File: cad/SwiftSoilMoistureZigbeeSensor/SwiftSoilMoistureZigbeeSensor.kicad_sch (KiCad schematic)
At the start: 12 parts, among them J1 Probe, J2 BAT, J3 TagConnect, Q1 BSS84, SW1 Factory Reset, U1 TPS61221DCK, U2 E73-2G4M08S1C

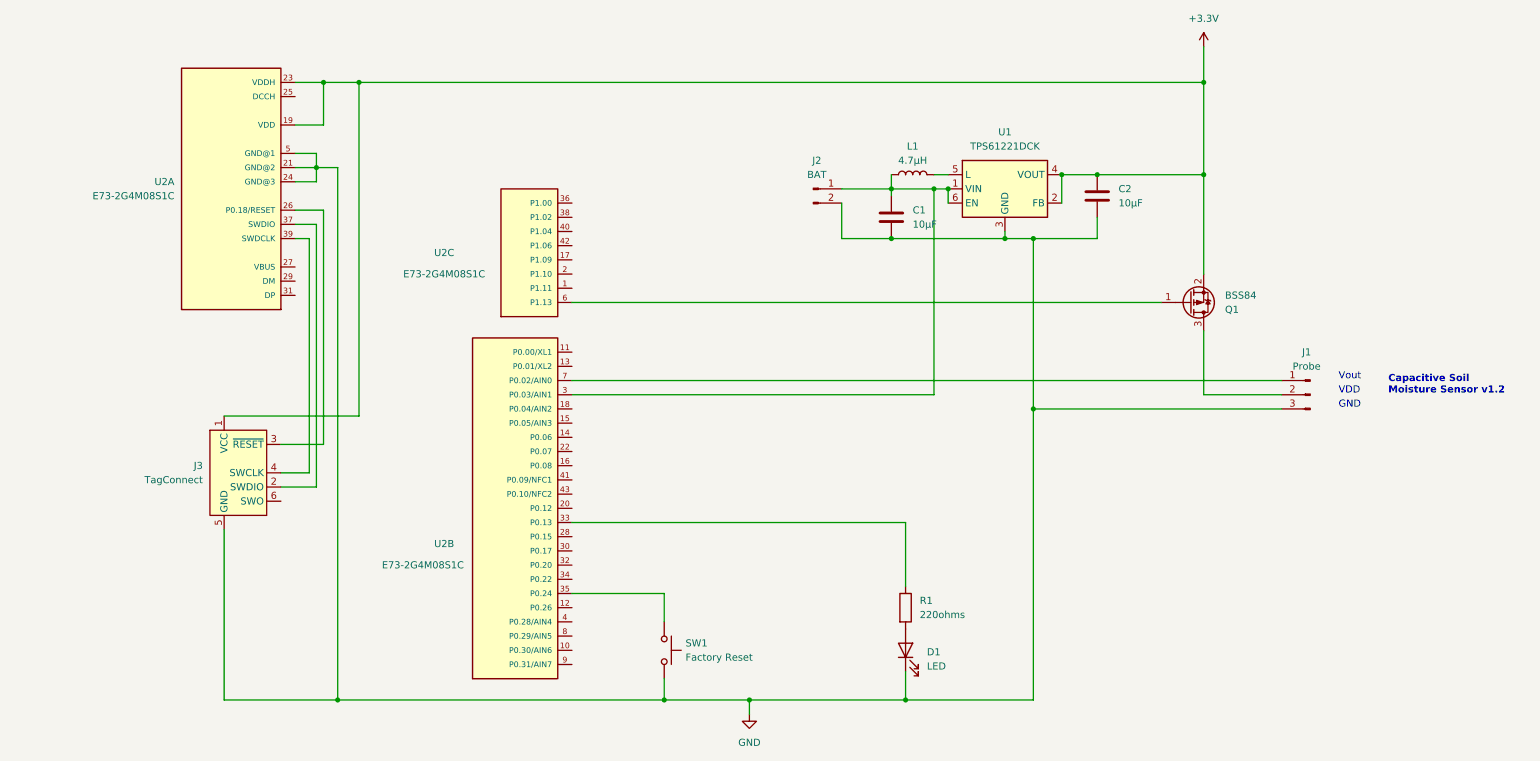
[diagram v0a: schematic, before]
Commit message: CAD Stuff
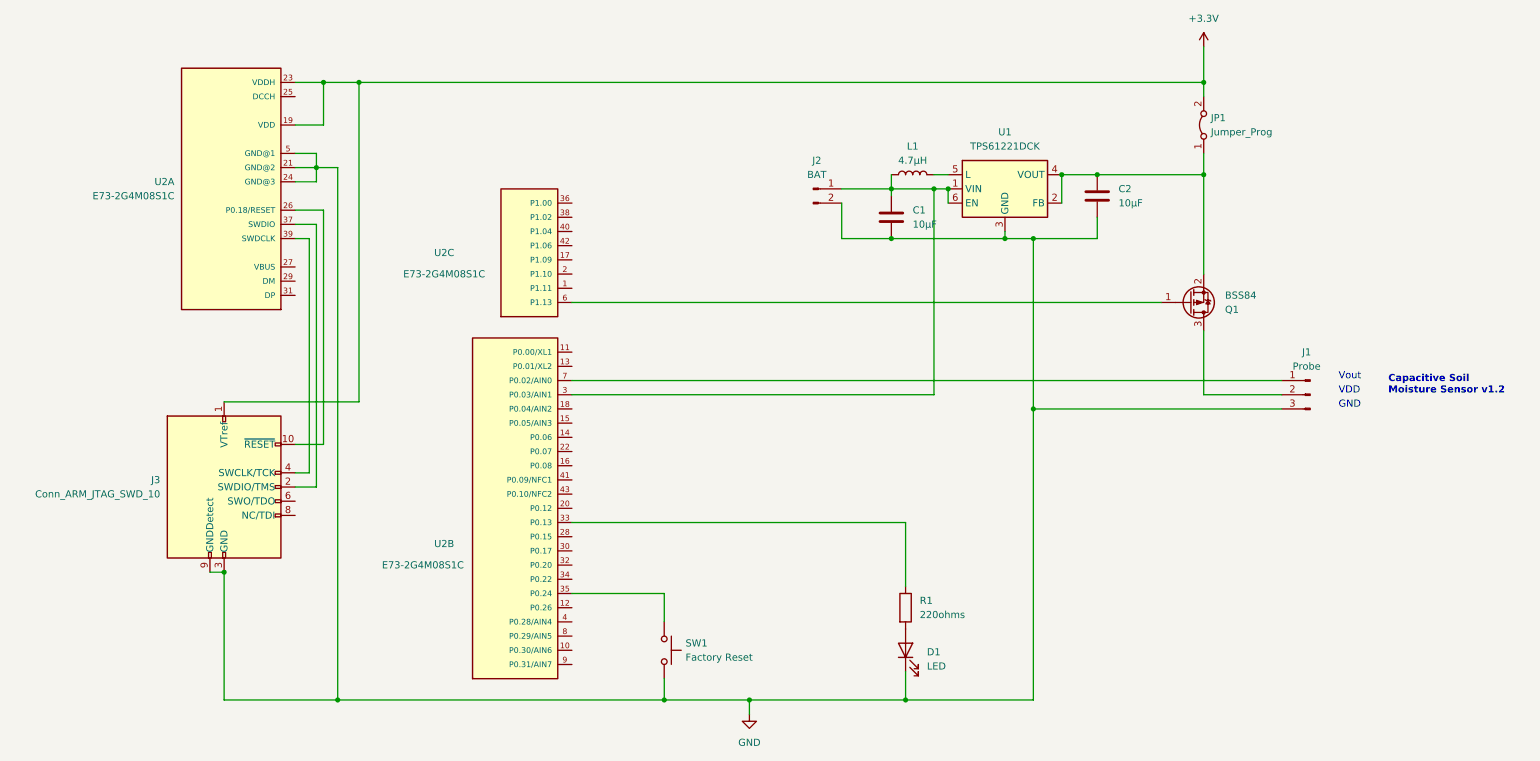
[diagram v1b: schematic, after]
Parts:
- removed J3: TagConnect, Connector:Tag-Connect_TC2030-IDC-NL_2x03_P1.27mm_Vertical, symbol Connector:Conn_ARM_SWD_TagConnect_TC2030-NL
- added J3: Conn_ARM_JTAG_SWD_10, Connector_PinHeader_1.27mm:PinHeader_2x05_P1.27mm_Vertical_SMD, symbol Connector:Conn_ARM_JTAG_SWD_10
- added JP1: Jumper_Prog, Connector_PinHeader_2.54mm:PinHeader_1x02_P2.54mm_Vertical, symbol Jumper:Jumper_2_Bridged
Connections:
- net +3.3V: now also J3.1 (VTref), JP1.2 (B); no longer C2.1, Q1.2 (S), U1.2 (FB), U1.4 (VOUT)
- net GND: now also J3.3 (GND), J3.5 (GND), J3.9 (GNDDetect)
- net at U2.26 (P0.18/RESET): now also J3.10 (~{RESET})
- net at U2.37 (SWDIO): now also J3.2 (SWDIO/TMS)
- net at U2.39 (SWDCLK): now also J3.4 (SWCLK/TCK)
- new net: C2.1, JP1.1 (A), Q1.2 (S), U1.2 (FB), U1.4 (VOUT)
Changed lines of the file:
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@@
   (junction (at 181.61 52.07) (diameter 0) (color 0 0 0 0)
   )
+  (junction (at 76.2 33.02) (diameter 0) (color 0 0 0 0)
+  )
+  (junction (at 171.45 52.07) (diameter 0) (color 0 0 0 0)
+  )
   (junction (at 227.33 49.53) (diameter 0) (color 0 0 0 0)
   )
-  (junction (at 76.2 33.02) (diameter 0) (color 0 0 0 0)
-  )
-  (junction (at 171.45 52.07) (diameter 0) (color 0 0 0 0)
-  )
   (junction (at 146.05 143.51) (diameter 0) (color 0 0 0 0)
   )
@@
   (junction (at 171.45 60.96) (diameter 0) (color 0 0 0 0)
   )
+  (junction (at 52.07 120.65) (diameter 0) (color 0 0 0 0)
+  )
   (junction (at 130.81 143.51) (diameter 0) (color 0 0 0 0)
   )
@@
   (junction (at 179.07 52.07) (diameter 0) (color 0 0 0 0)
   )
+  (junction (at 173.99 143.51) (diameter 0) (color 0 0 0 0)
+  )
+  (junction (at 191.77 60.96) (diameter 0) (color 0 0 0 0)
+  )
   (junction (at 227.33 33.02) (diameter 0) (color 0 0 0 0)
   )
-  (junction (at 173.99 143.51) (diameter 0) (color 0 0 0 0)
-  )
-  (junction (at 191.77 60.96) (diameter 0) (color 0 0 0 0)
+  (wire (pts (xy 52.07 120.65) (xy 49.53 120.65))
+    (stroke (width 0) (type default))
   )
   (wire (pts (xy 72.39 48.26) (xy 72.39 143.51))
@@
     (stroke (width 0) (type default))
   )
-  (wire (pts (xy 62.23 102.87) (xy 67.31 102.87))
+  (wire (pts (xy 64.77 102.87) (xy 67.31 102.87))
     (stroke (width 0) (type default))
   )
@@
     (stroke (width 0) (type default))
   )
-  (wire (pts (xy 227.33 33.02) (xy 227.33 49.53))
-    (stroke (width 0) (type default))
-  )
-  (wire (pts (xy 62.23 105.41) (xy 68.58 105.41))
+  (wire (pts (xy 64.77 105.41) (xy 68.58 105.41))
     (stroke (width 0) (type default))
   )
@@
     (stroke (width 0) (type default))
   )
-  (wire (pts (xy 52.07 113.03) (xy 52.07 143.51))
+  (wire (pts (xy 227.33 45.72) (xy 227.33 49.53))
+    (stroke (width 0) (type default))
+  )
+  (wire (pts (xy 227.33 33.02) (xy 227.33 35.56))
     (stroke (width 0) (type default))
   )
@@
     (stroke (width 0) (type default))
   )
+  (wire (pts (xy 52.07 120.65) (xy 52.07 143.51))
+    (stroke (width 0) (type default))
+  )
   (wire (pts (xy 171.45 49.53) (xy 171.45 52.07))
     (stroke (width 0) (type default))
@@
     (stroke (width 0) (type default))
   )
-  (wire (pts (xy 76.2 92.71) (xy 76.2 33.02))
+  (wire (pts (xy 76.2 90.17) (xy 76.2 33.02))
     (stroke (width 0) (type default))
   )
@@
     (stroke (width 0) (type default))
   )
-  (wire (pts (xy 52.07 92.71) (xy 76.2 92.71))
+  (wire (pts (xy 52.07 90.17) (xy 76.2 90.17))
     (stroke (width 0) (type default))
   )
@@
     (stroke (width 0) (type default))
   )
-  (wire (pts (xy 64.77 55.88) (xy 69.85 55.88))
+  (wire (pts (xy 69.85 55.88) (xy 64.77 55.88))
     (stroke (width 0) (type default))
   )
@@
     (stroke (width 0) (type default))
   )
-  (wire (pts (xy 62.23 97.79) (xy 69.85 97.79))
+  (wire (pts (xy 64.77 97.79) (xy 69.85 97.79))
     (stroke (width 0) (type default))
   )
@@
     )
   )
+  (symbol (lib_id "Jumper:Jumper_2_Bridged") (at 227.33 40.64 90) (unit 1)
+    (in_bom yes) (on_board yes) (dnp no) (fields_autoplaced)
+    (property "Reference" "JP1" (at 228.6 39.37 90)
+      (effects (font (size 1.27 1.27)) (justify right))
+    )
+    (property "Value" "Jumper_Prog" (at 228.6 41.91 90)
+      (effects (font (size 1.27 1.27)) (justify right))
+    )
+    (property "Footprint" "Connector_PinHeader_2.54mm:PinHeader_1x02_P2.54mm_Vertical" (at 227.33 40.64 0)
+      (effects (font (size 1.27 1.27)) hide)
+    )
+    (property "Datasheet" "~" (at 227.33 40.64 0)
+      (effects (font (size 1.27 1.27)) hide)
+    )
+    (pin "1")
+    (pin "2")
+    (instances
+      (project "SwiftSoilMoistureZigbeeSensor"
+        (path "/abcc6947-5804-4900-9240-6fa6b27c7542"
+          (reference "JP1") (unit 1)
+        )
+      )
+    )
+  )
+  (symbol (lib_id "Connector:Conn_ARM_JTAG_SWD_10") (at 52.07 105.41 0) (unit 1)
+    (in_bom yes) (on_board yes) (dnp no) (fields_autoplaced)
+    (property "Reference" "J3" (at 40.64 104.14 0)
+      (effects (font (size 1.27 1.27)) (justify right))
+    )
+    (property "Value" "Conn_ARM_JTAG_SWD_10" (at 40.64 106.68 0)
+      (effects (font (size 1.27 1.27)) (justify right))
+    )
+    (property "Footprint" "Connector_PinHeader_1.27mm:PinHeader_2x05_P1.27mm_Vertical_SMD" (at 52.07 105.41 0)
+      (effects (font (size 1.27 1.27)) hide)
+    )
+    (property "Datasheet" "http://infocenter.arm.com/help/topic/com.arm.doc.ddi0314h/DDI0314H_coresight_components_trm.pdf" (at 43.18 137.16 90)
+      (effects (font (size 1.27 1.27)) hide)
+    )
+    (pin "5")
+    (pin "2")
+    (pin "3")
+    (pin "4")
+    (pin "6")
+    (pin "10")
+    (pin "1")
+    (pin "7")
+    (pin "9")
+    (pin "8")
+    (instances
+      (project "SwiftSoilMoistureZigbeeSensor"
+        (path "/abcc6947-5804-4900-9240-6fa6b27c7542"
+          (reference "J3") (unit 1)
+        )
+      )
+    )
+  )
   (symbol (lib_id "power:+3.3V") (at 227.33 26.67 0) (unit 1)
     (in_bom yes) (on_board yes) (dnp no) (fields_autoplaced)
@@
         )
       )
-    )
-  )
-  (symbol (lib_id "Connector:Conn_ARM_SWD_TagConnect_TC2030-NL") (at 54.61 102.87 0) (unit 1)
-    (in_bom no) (on_board yes) (dnp no) (fields_autoplaced)
-    (property "Reference" "J3" (at 48.26 101.6 0)
-      (effects (font (size 1.27 1.27)) (justify right))
-    )
-    (property "Value" "TagConnect" (at 48.26 104.14 0)
-      (effects (font (size 1.27 1.27)) (justify right))
-    )
-    (property "Footprint" "Connector:Tag-Connect_TC2030-IDC-NL_2x03_P1.27mm_Vertical" (at 54.61 120.65 0)
-      (effects (font (size 1.27 1.27)) hide)
-    )
-    (property "Datasheet" "https://www.tag-connect.com/wp-content/uploads/bsk-pdf-manager/TC2030-CTX_1.pdf" (at 54.61 118.11 0)
-      (effects (font (size 1.27 1.27)) hide)
-    )
-    (pin "5")
-    (pin "3")
-    (pin "4")
-    (pin "6")
-    (pin "1")
-    (pin "2")
-    (instances
-      (project "SwiftSoilMoistureZigbeeSensor"
-        (path "/abcc6947-5804-4900-9240-6fa6b27c7542"
-          (reference "J3") (unit 1)
-        )
-      )
